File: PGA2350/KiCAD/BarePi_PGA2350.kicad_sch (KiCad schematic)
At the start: 15 parts, among them J1 OUT, J2 DISPLAY, J3 USB, SW1 BOOTSEL, U1 PGA2350

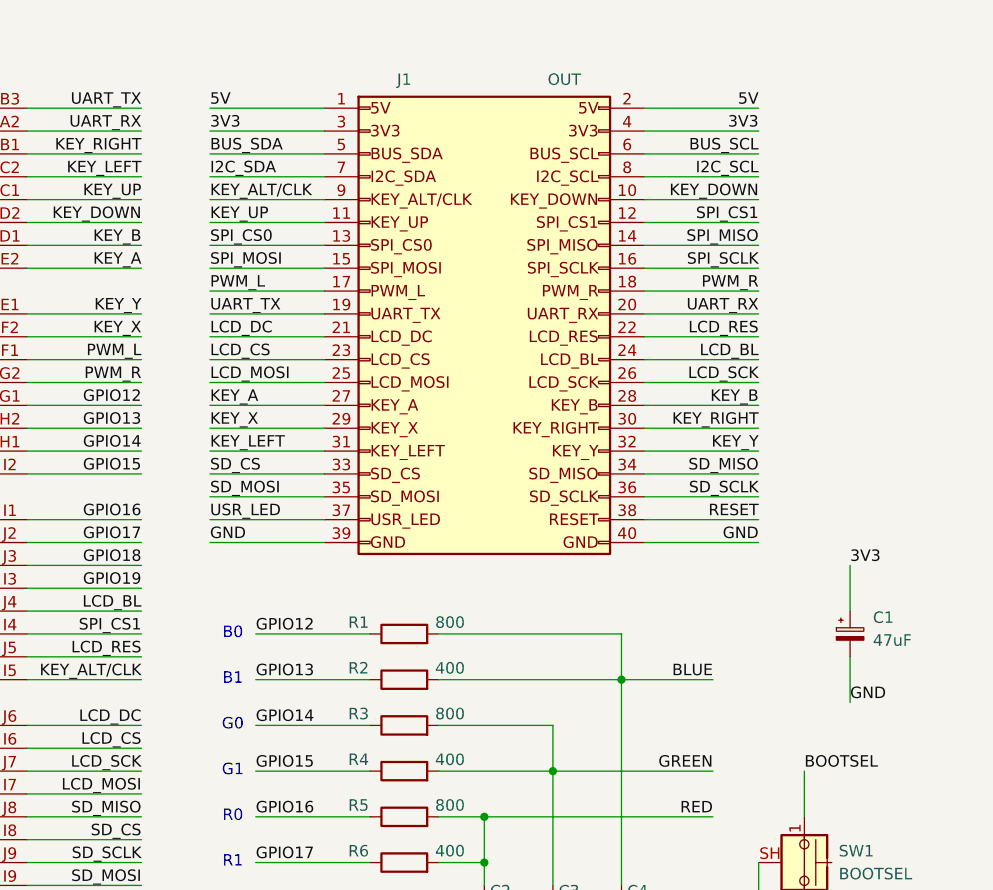
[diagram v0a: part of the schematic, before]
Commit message: init
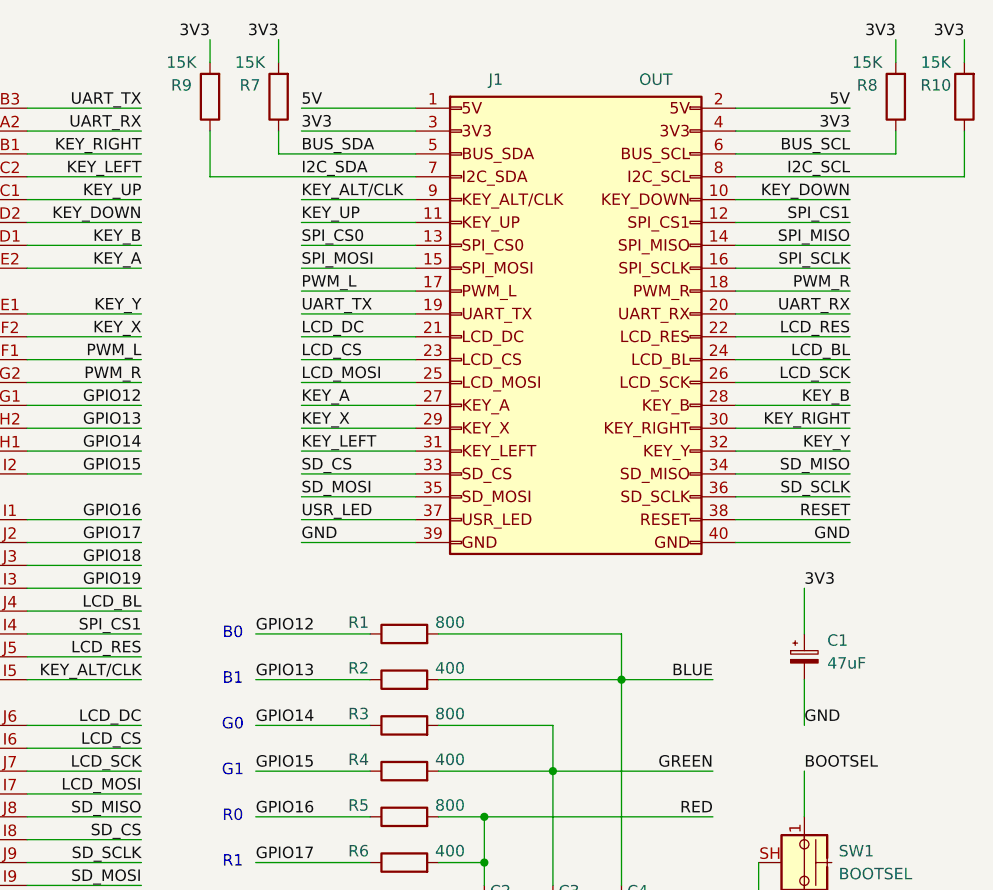
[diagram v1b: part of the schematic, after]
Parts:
- added R10, R7, R8, R9: 15K, Resistor_SMD:R_1206_3216Metric_Pad1.30x1.75mm_HandSolder, symbol Device:R
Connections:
- net 3V3: now also R10.2, R7.2, R8.2, R9.2
- net BUS_SCL: now also R8.1
- net BUS_SDA: now also R7.1
- net I2C_SCL: now also R10.1
- net I2C_SDA: now also R9.1
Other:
- moved on the sheet: C1, J1
